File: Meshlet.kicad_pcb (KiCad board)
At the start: 4 copper layers, 42.5 x 32 mm, 97 parts, among them J13 Thermistor Pins, J14 Ext. Notif. Header, J2 User Btn Header, J3 Batt. Header (Picoblade 1.25), J4 Batt. Header (JST-PH 2.0), J5 USB_C_Receptacle_USB2.0_16P, J6 STEMMA QT I2C, J7 Ext. Power Header, J9 Ext. Power Header, Q1 AO3400A, SW2 BOOTSEL, U1 XC6206PxxxMR, U11 INA3221, U2 USBLC6-2SC6, U3 XC6206PxxxMR, U4 RP2350_60QFN, U5 Wio-SX1262, U6 BQ25185, U7 BME280, U8 W25Q32JVZP, U9 XC6206PxxxMR, Y1 12.000MHz

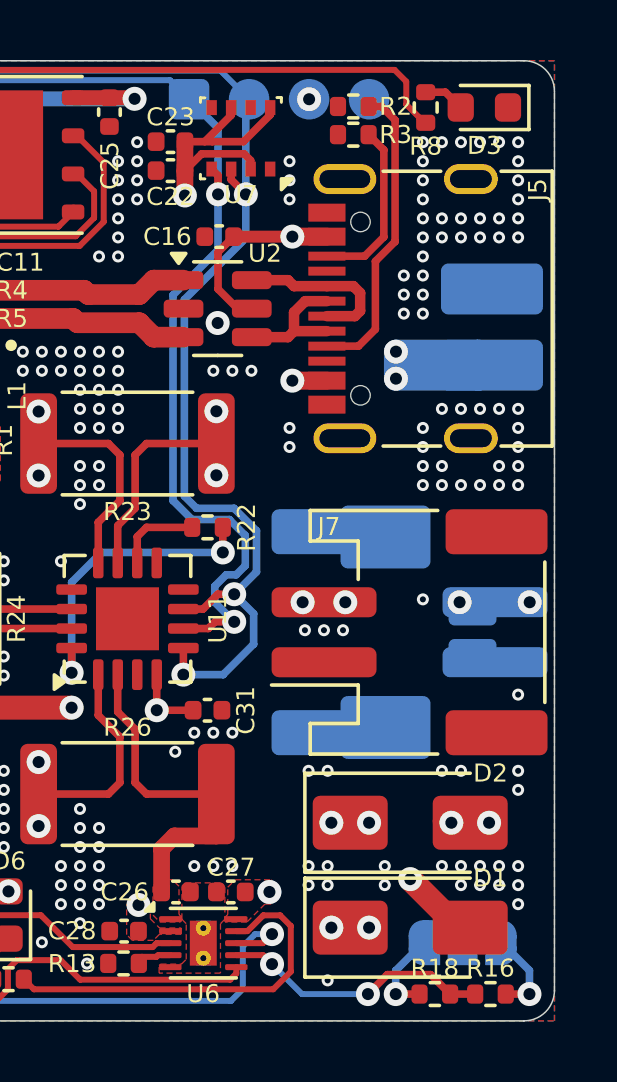
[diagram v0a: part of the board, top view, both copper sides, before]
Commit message: Small changes
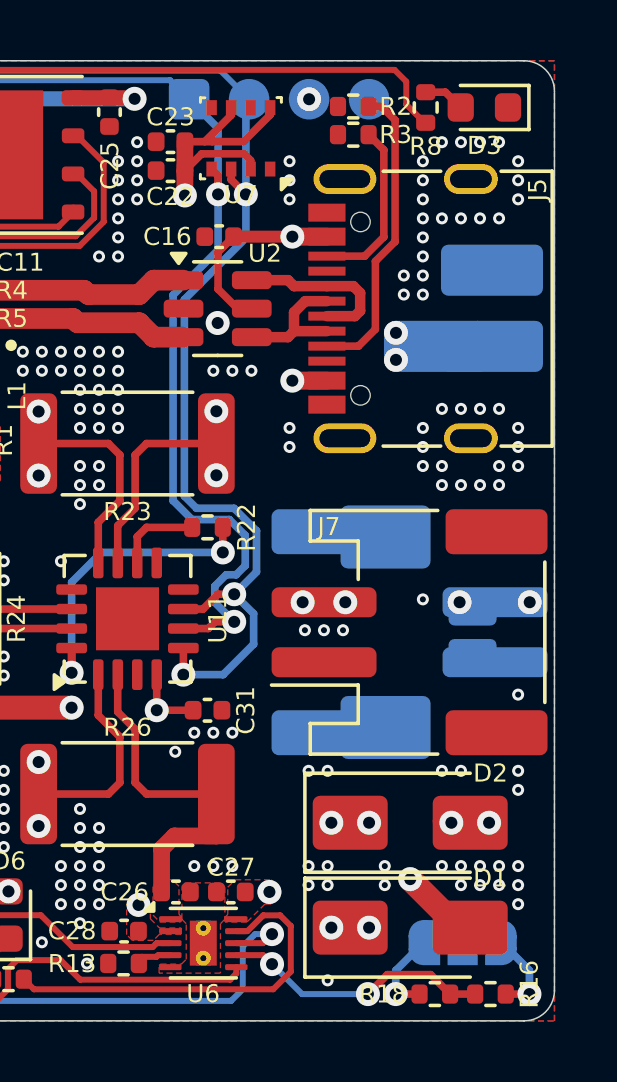
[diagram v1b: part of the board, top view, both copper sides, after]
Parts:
- moved J9 0.63 mm to (162.9, 85.5)
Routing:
- net GND: vias 336 -> 323
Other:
- board text added: "NETWORK NODE RP2350 MESH NETWORK NODE RP2350 MESH NETWORK NODE"
- board text removed: "RP2350 MESH NETWORK NODE RP2350 MESH NETWORK NODE"
